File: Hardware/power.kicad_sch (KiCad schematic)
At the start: 67 parts, among them J4 Barrel_Jack_Switch, U1 STM32MP157FAD1, U2 STPMIC1

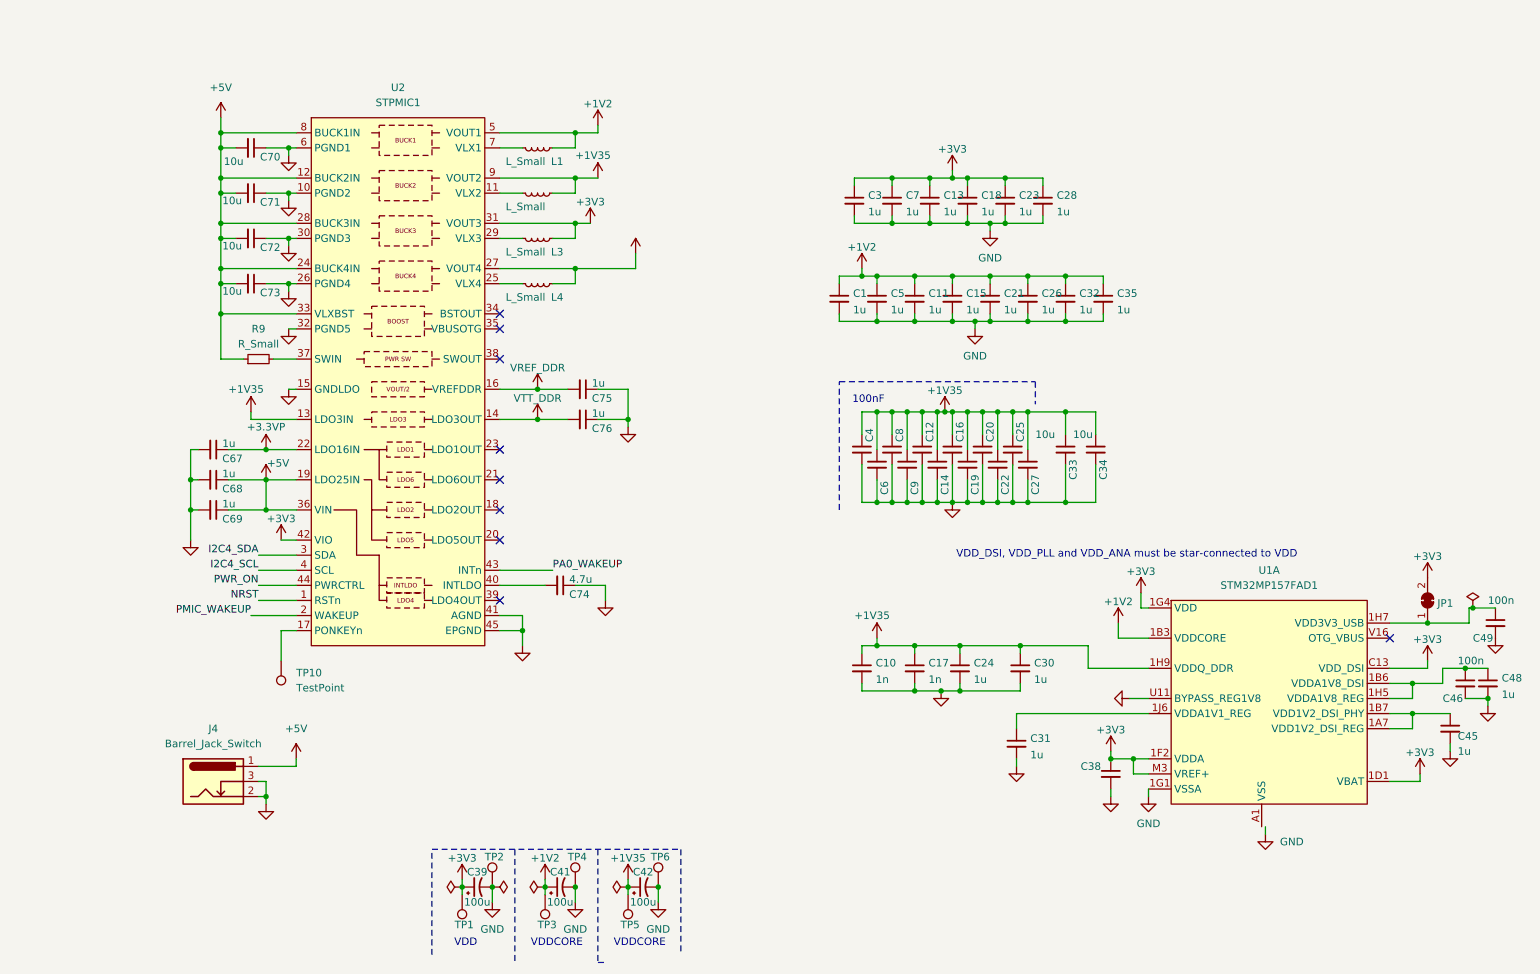
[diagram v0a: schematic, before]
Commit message: First Draft schematic (R2)
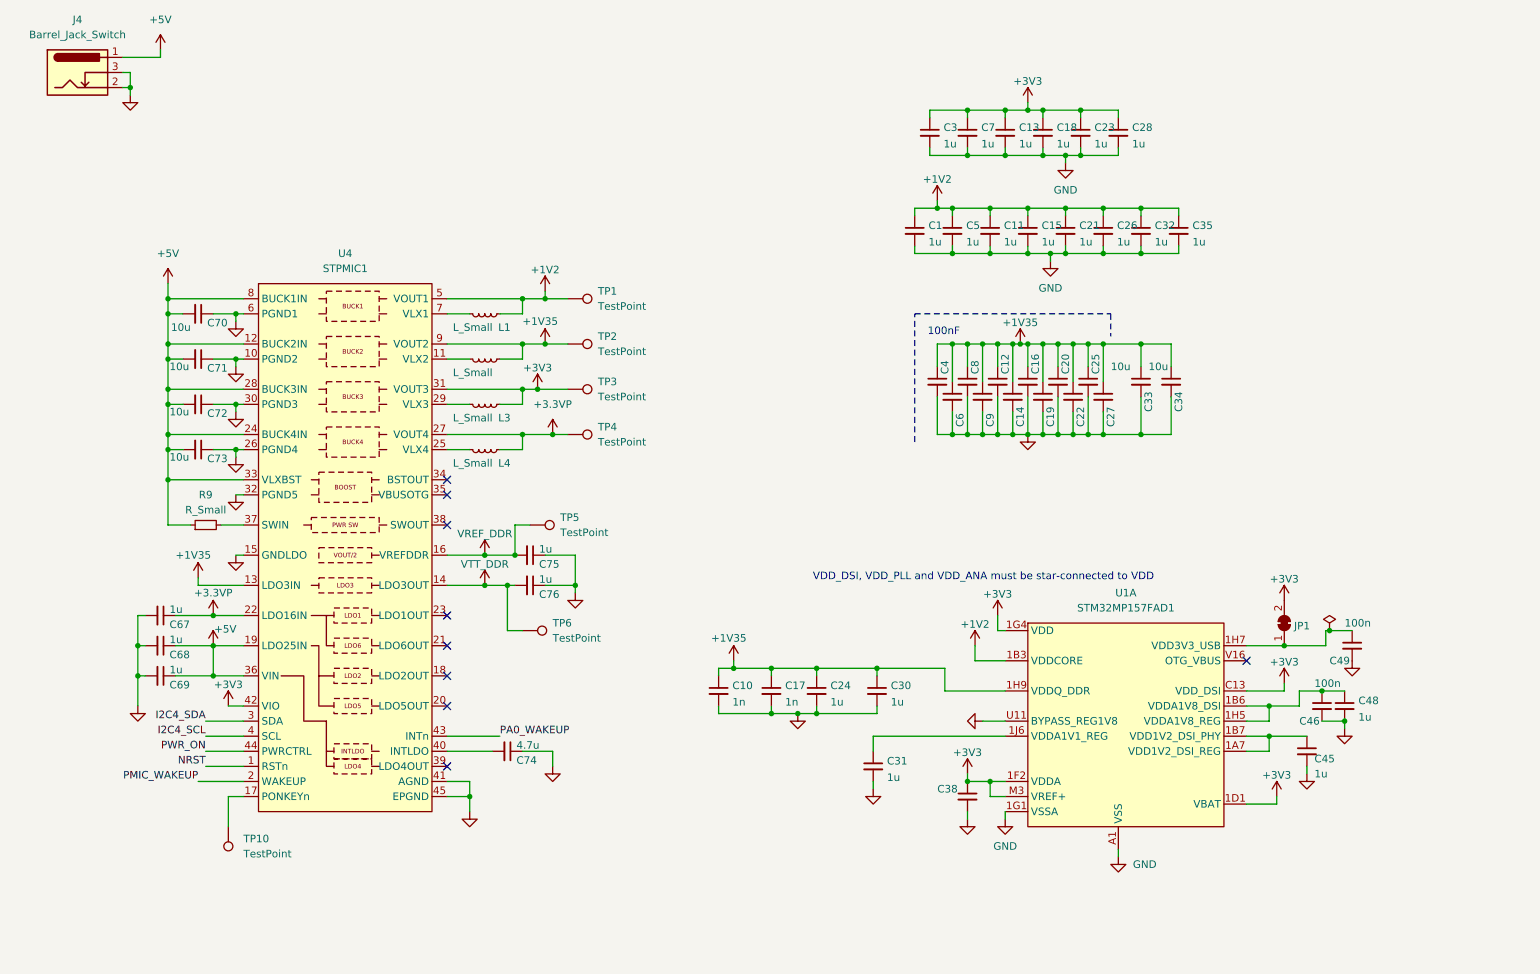
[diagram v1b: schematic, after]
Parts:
- removed C39, C41, C42: 100u, Capacitor_SMD:C_1206_3216Metric, symbol Device:C_Polarized_Small_US
- removed U2: STPMIC1, BioMEMS:WFQFN44L, symbol SimpleSBC:STPMIC1APQR
- added U4: STPMIC1, SimpleSBC:WFQFN44L, symbol SimpleSBC:STPMIC1APQR
- TP1, TP2, TP3, TP4, TP5, TP6: value TestPoint-SP -> TestPoint; footprint personal:PROBE_PAD_1206 -> (none)
- U1: footprint personal:TFBGA257 -> SimpleSBC:TFBGA257
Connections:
- net VSS is gone; now on net GND: U1.1A6 (VSS), U1.1B8 (VSS), U1.1C3 (VSS), U1.1C5 (VSS), U1.1C7 (VSS), U1.1D2 (VSS), U1.1D4 (VSS), U1.1D6 (VSS), U1.1E3 (VSS), U1.1E5 (VSS), U1.1E7 (VSS), U1.1F4 (VSS), U1.1F6 (VSS), U1.1G2 (VSS), U1.1G5 (VSS), U1.1G7 (VSS), U1.1H2 (VSS), U1.1H3 (VSS), U1.1H4 (VSS), U1.1H6 (VSS), U1.1H8 (VSS), U1.1J5 (VSS), U1.1J9 (VSS), U1.A1 (VSS), U1.A19 (VSS), U1.A6 (VSS), U1.C14 (VSS), U1.D17 (VSS), U1.F18 (VSS), U1.F3 (VSS), U1.G1 (VSS), U1.G17 (VSS), U1.K17 (VSS), U1.K19 (VSS), U1.N1 (VSS), U1.N17 (VSS), U1.R19 (VSS), U1.U9 (VSS), U1.W1 (VSS), U1.W13 (VSS), U1.W19 (VSS), U1.W5 (VSS)
- net +1V2: now also TP1.1, U4.5 (VOUT1); no longer TP3.1
- net +1V35: now also TP2.1, U4.13 (LDO3IN), U4.9 (VOUT2); no longer TP5.1
- net +3.3VP: now also TP4.1, U4.22 (LDO16IN), U4.27 (VOUT4)
- net +3V3: now also TP3.1, U4.31 (VOUT3), U4.42 (VIO); no longer TP1.1
- net +5V: now also U4.12 (BUCK2IN), U4.19 (LDO25IN), U4.24 (BUCK4IN), U4.28 (BUCK3IN), U4.33 (VLXBST), U4.36 (VIN), U4.8 (BUCK1IN)
- net GND: now also U4.10 (PGND2), U4.15 (GNDLDO), U4.26 (PGND4), U4.30 (PGND3), U4.32 (PGND5), U4.41 (AGND), U4.45 (EPGND), U4.6 (PGND1); no longer TP2.1, TP4.1, TP6.1
- net I2C4_SCL: now also U4.4 (SCL)
- net I2C4_SDA: now also U4.3 (SDA)
- net NRST: now also U4.1 (RSTn)
- net PA0_WAKEUP: now also U4.43 (INTn)
- net PMIC_WAKEUP: now also U4.2 (WAKEUP)
- net PWR_ON: now also U4.44 (PWRCTRL)
- net VREF_DDR: now also TP5.1, U4.16 (VREFDDR)
- net VTT_DDR: now also TP6.1, U4.14 (LDO3OUT)
- net at L2.1: now also U4.11 (VLX2)
- net at R9.2: now also U4.37 (SWIN)
- net at C74.2: now also U4.40 (INTLDO)
- net at TP10.1: now also U4.17 (PONKEYn)
- net at L3.1: now also U4.29 (VLX3)
- net at L4.1: now also U4.25 (VLX4)
- net at L1.1: now also U4.7 (VLX1)
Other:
- note removed: "VDD"
- note removed: "VDDCORE"
- title: (none) -> SimpleSBC Power
- moved on the sheet: C1, C10, C11, C12, C13, C14, C15, C16, C17, C18, C19, C20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
